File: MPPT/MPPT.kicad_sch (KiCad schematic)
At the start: 49 parts, among them U1 TPS7H4010MRNPTSEP, U2 5962L1620901VYC, U3 5962L1620901VYC, U4 5962L1620901VYC, U5 5962L1620901VYC, U6 5962L1620901VYC, U7 5962L1620901VYC

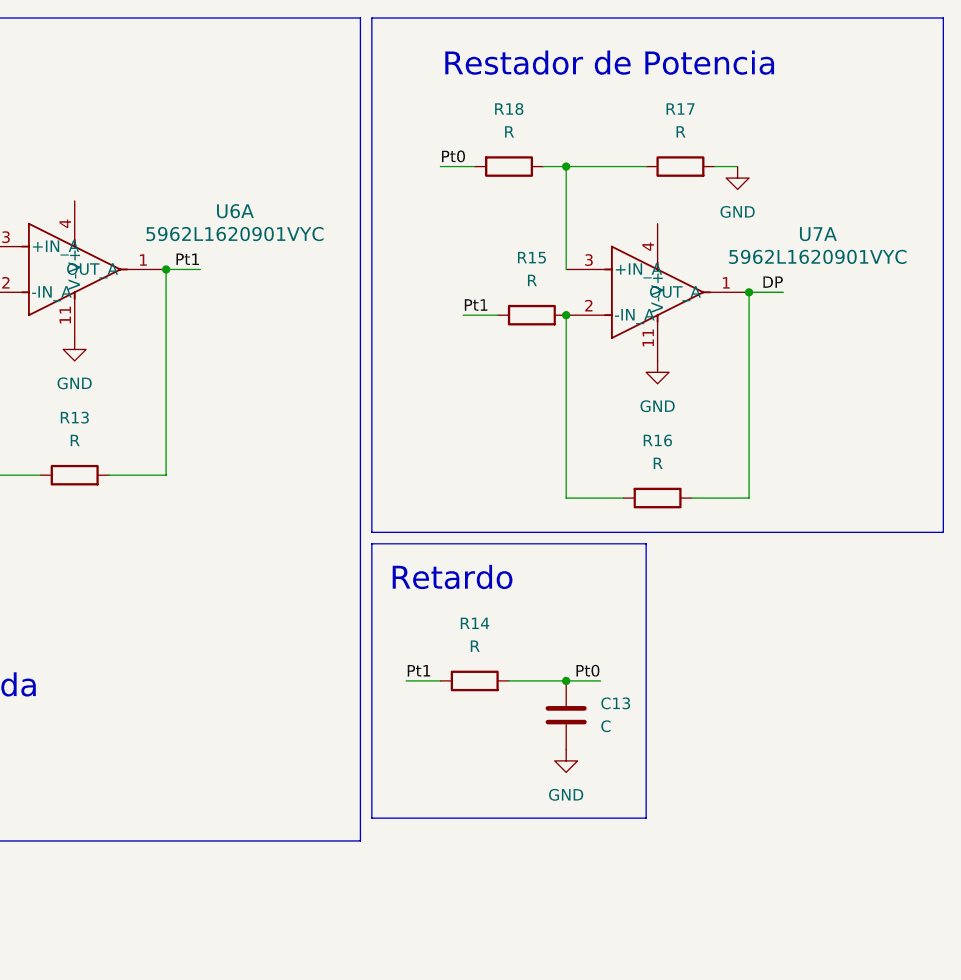
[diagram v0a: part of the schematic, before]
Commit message: Se crea el restador y un retardo de la potencia
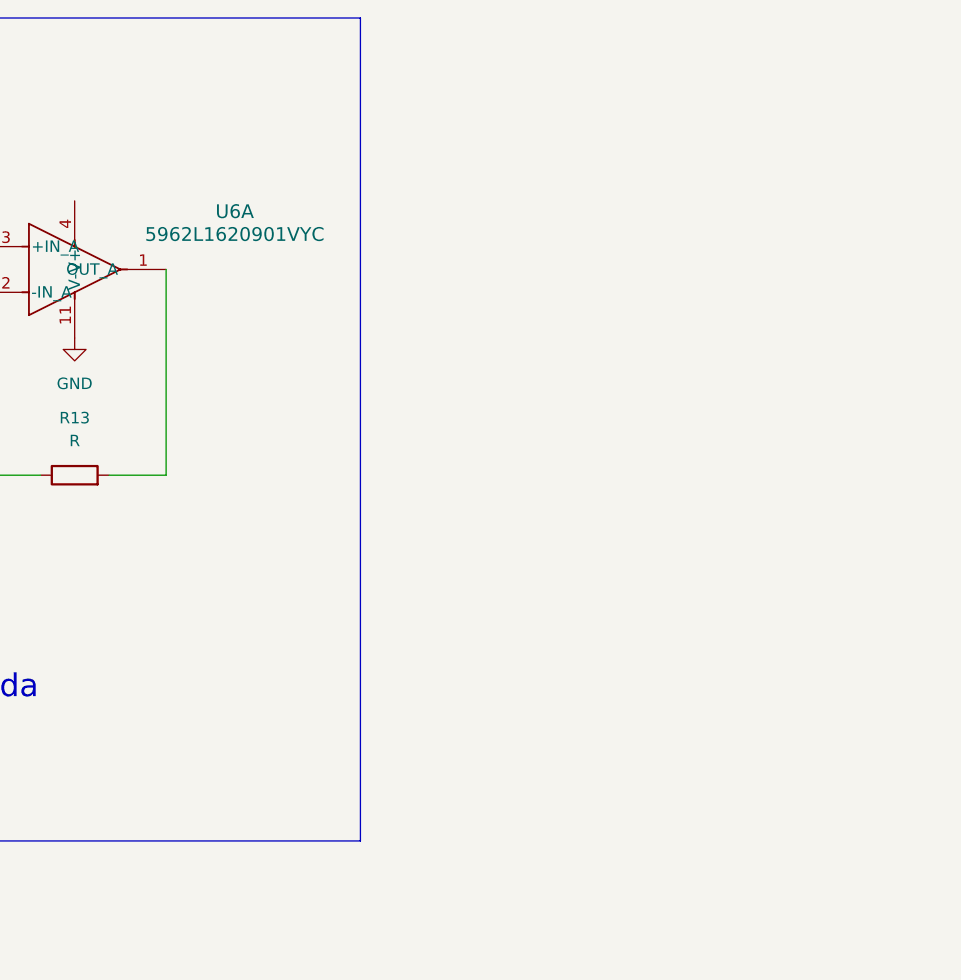
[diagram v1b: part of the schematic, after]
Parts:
- removed C13: C, symbol Device:C
- removed R14, R15, R16, R17, R18: R, symbol Device:R
- removed U7: 5962L1620901VYC, HFR0014A-IPC_A, symbol 5962L1620901VYC:5962L1620901VYC
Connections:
- net Pt1: no longer names the net of R13.2, U6.1 (OUT_A)
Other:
- note removed: "Restador de Potencia"
- note removed: "Retardo"

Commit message: Create ~MPPT.kicad_sch.lck
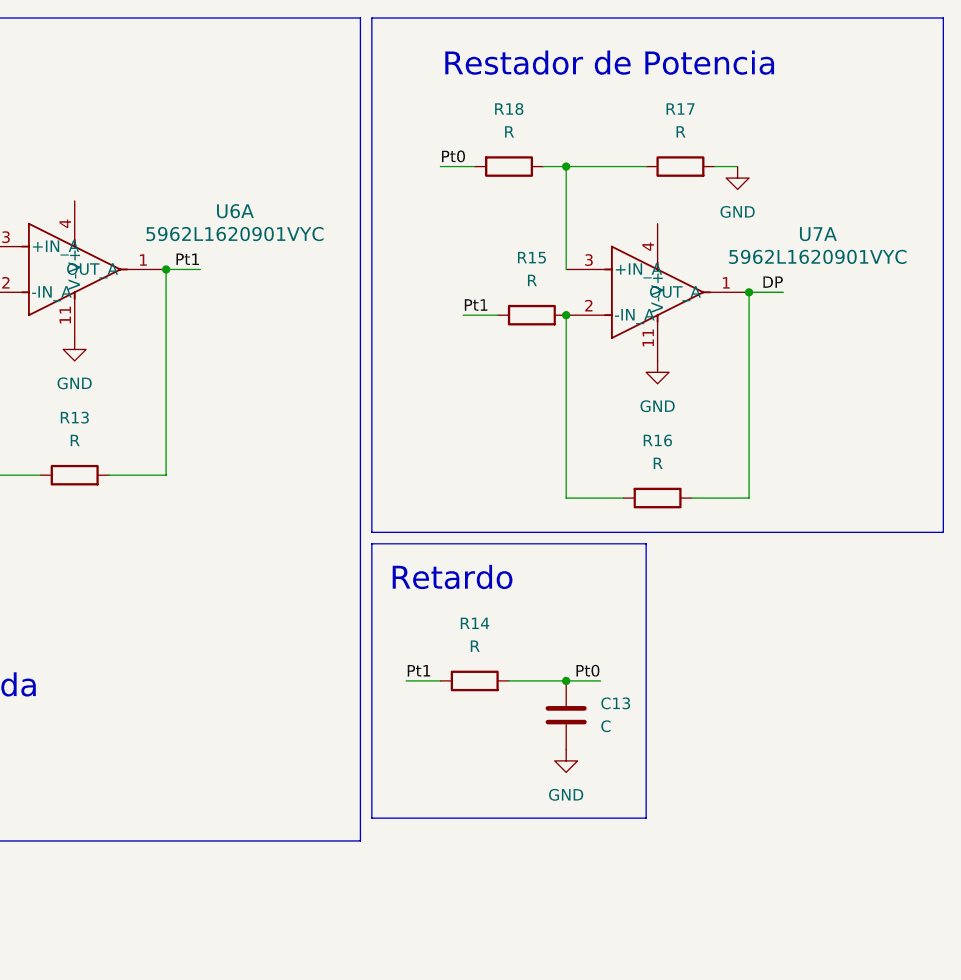
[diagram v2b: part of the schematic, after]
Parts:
- added C13: C, symbol Device:C
- added R14, R15, R16, R17, R18: R, symbol Device:R
- added U7: 5962L1620901VYC, HFR0014A-IPC_A, symbol 5962L1620901VYC:5962L1620901VYC
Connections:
- net GND: now also C13.2, R17.2, U7.11 (V-)
- net Pt1: now reaches R13.2, U6.1 (OUT_A)
- net Pt1: now also R14.1, R15.1
- new net: R15.2, R16.2, U7.2 (-IN_A)
- new net: R17.1, R18.1, U7.3 (+IN_A)
- new net DP: R16.1, U7.1 (OUT_A)
- new net Pt0: C13.1, R14.2, R18.2
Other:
- note added: "Restador de Potencia"
- note added: "Retardo"
